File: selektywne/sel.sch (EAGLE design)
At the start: 126 parts, among them IC1 TPS70925DBVT, IC2 SP3485EN-L_TR, J1 5-1634556-0, J2 5-1634556-0, J3 5-1634556-0, J4 5-1634556-0, J6 5-1634556-0, J7 5-1634556-0, J8 5-1634556-0, U1 ADS1248IPW, U3 TLC274CN, U4 TPS72301DBVT, U6 TLC274CN, U7 TLC274CN, X2 0446200002

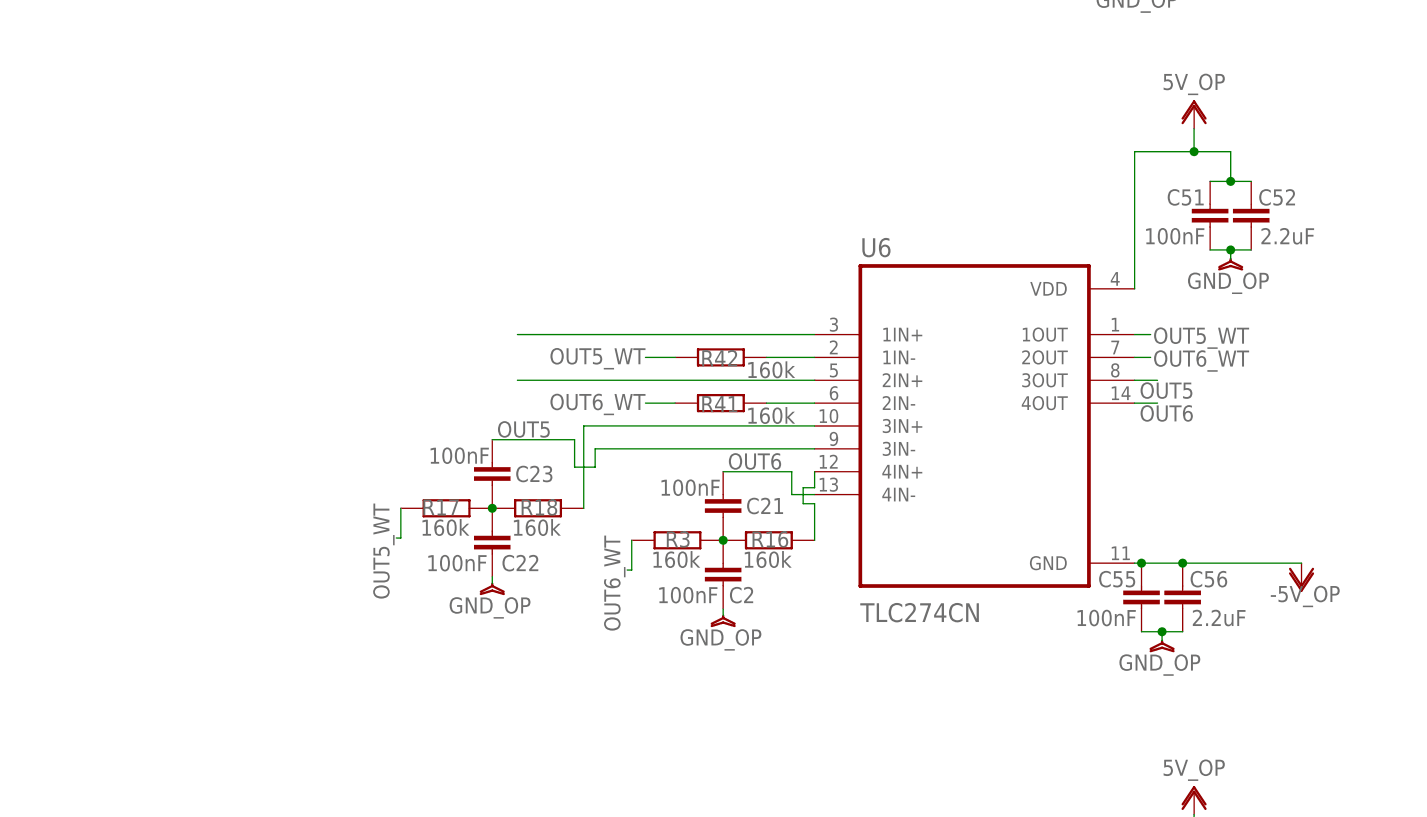
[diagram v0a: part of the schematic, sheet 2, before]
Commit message: fux wt problem
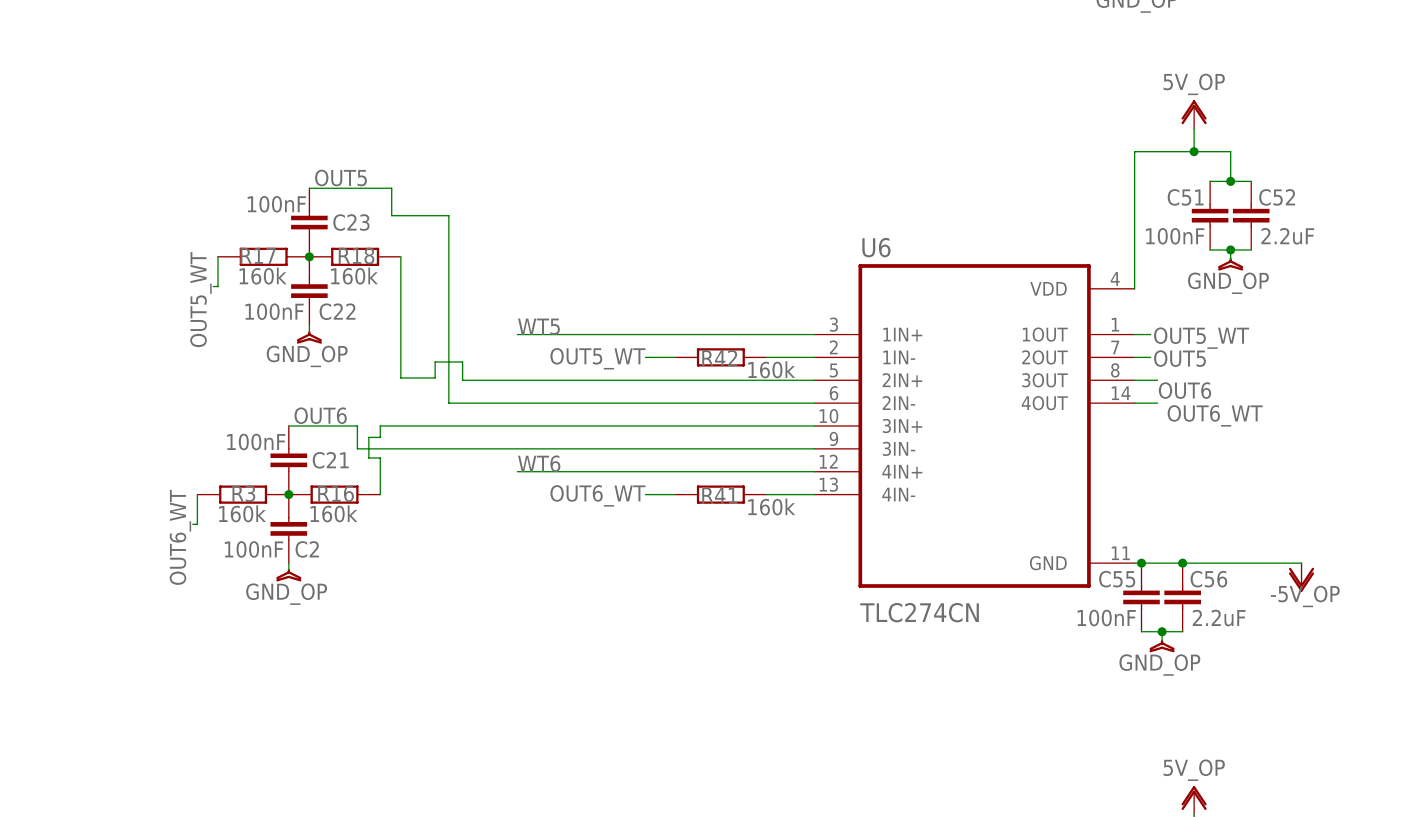
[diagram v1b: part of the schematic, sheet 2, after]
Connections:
- net 1IN+_2 renamed WT5
- removed net 2IN+_2: U6.2IN+
- removed net 4IN+_2: R16.1, U6.4IN+
- removed net N$27: R41.1, U6.2IN-
- new net 3IN+_2: R16.1, U6.3IN+
- new net N$1: R41.1, U6.4IN-
- new net WT6: U6.4IN+
- net N$3: now also U6.2IN+; no longer U6.3IN+
- net OUT5: now also U6.2IN-, U6.2OUT; no longer U6.3IN-, U6.3OUT
- net OUT6: now also U6.3IN-, U6.3OUT; no longer U6.4IN-, U6.4OUT
- net OUT6_WT: now also U6.4OUT; no longer U6.2OUT
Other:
- moved on the sheet: C2, C21, C22, C23, R16, R17, R18, R3, R41
